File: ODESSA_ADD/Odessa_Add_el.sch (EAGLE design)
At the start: 18 parts, among them SW2 ВЫКЛ., SW3 ВКЛ., SW4 ВКЛ., SW5 ВЫКЛ.

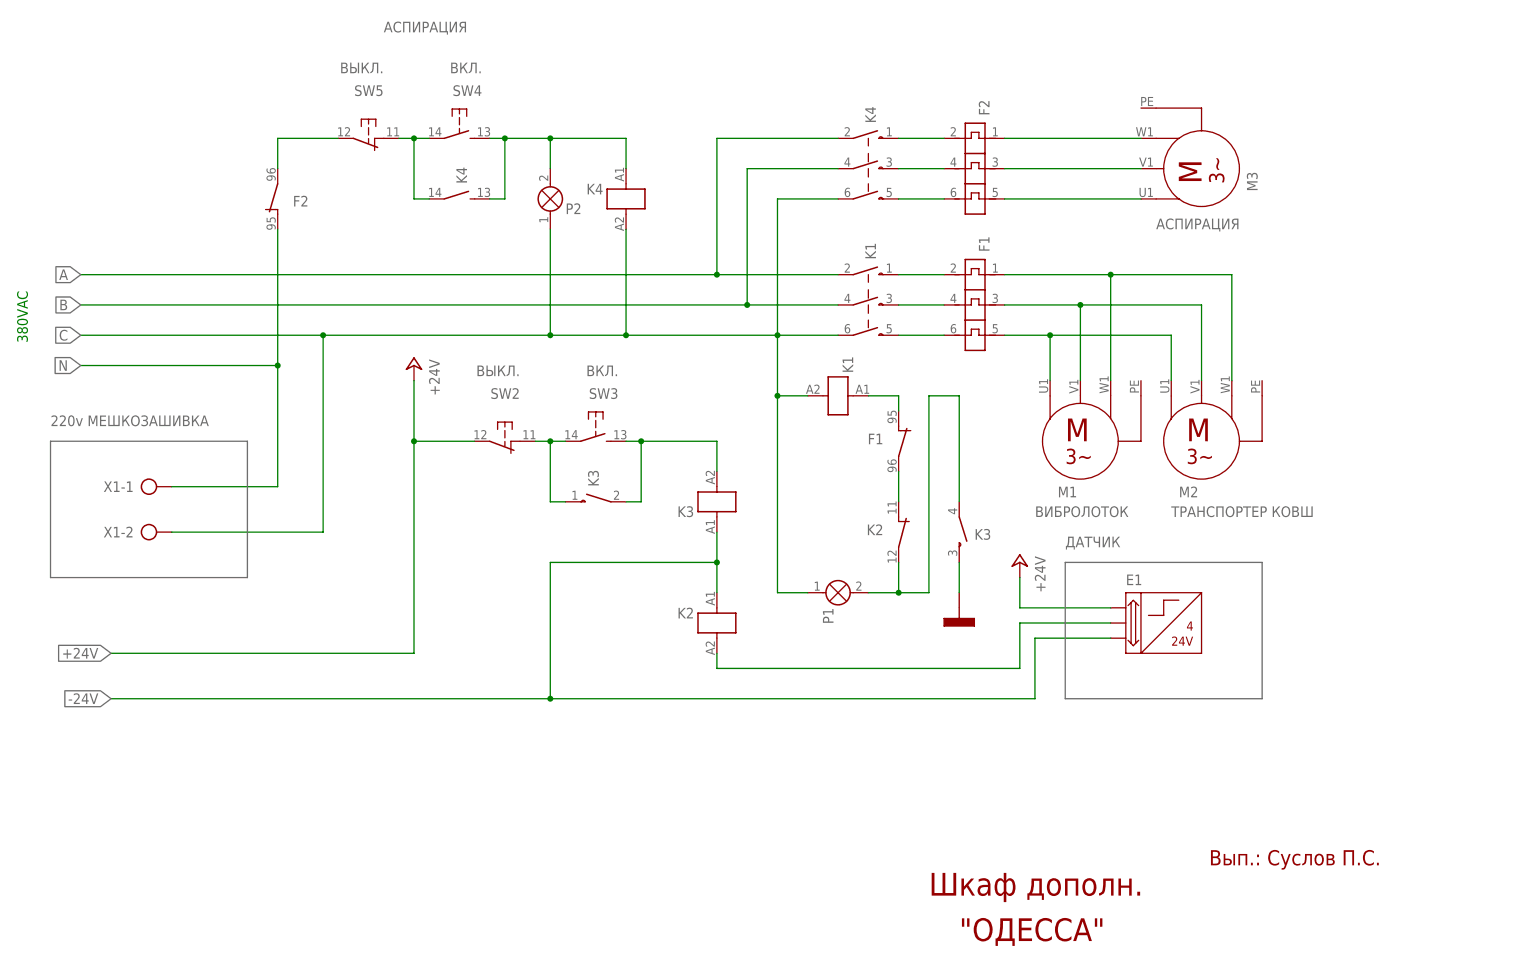
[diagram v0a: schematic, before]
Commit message: ODESSA
fix something
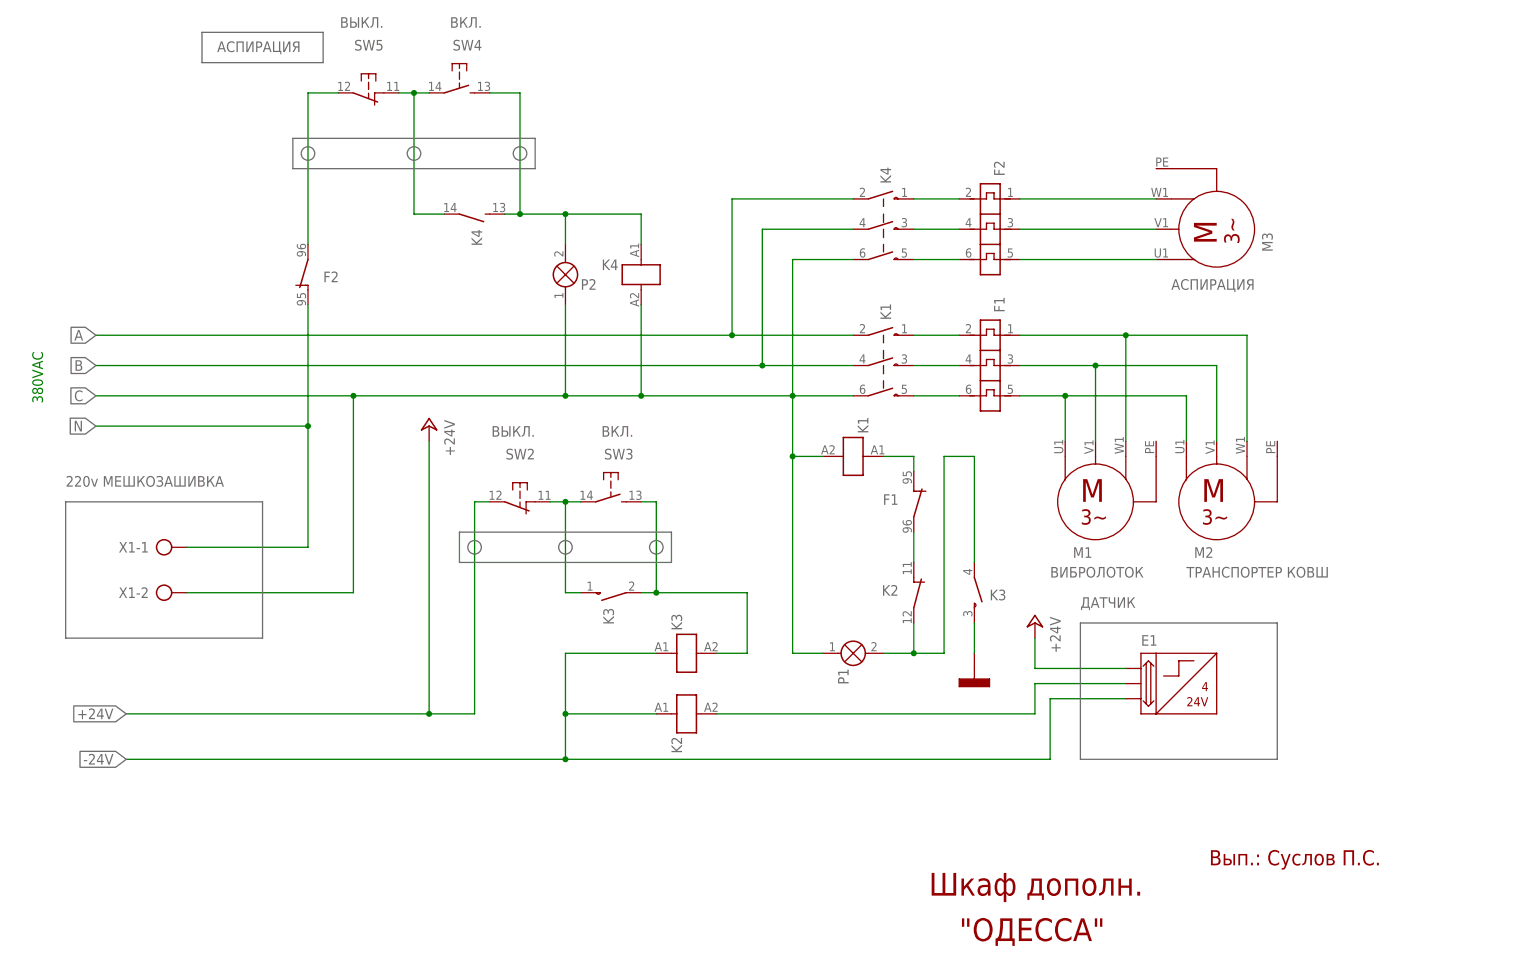
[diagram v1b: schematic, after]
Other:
- moved on the sheet: E1, F1, F2, K1, K2, K3, K4, M1, M2, M3, P1, P2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
